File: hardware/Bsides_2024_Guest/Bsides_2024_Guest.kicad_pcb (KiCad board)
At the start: 2 copper layers, 134.5 x 127.4 mm, 45 parts, among them J1 Conn_02x03_Odd_Even, J2 Battery, J3 Battery, J4 OLED, J5 Conn_01x05, J6 Conn_01x05, P1 USB_C_Plug_USB2.0, Q1 DMG3415U-7, SW1 ON, SW2 RESET, SW3 BOOT, SW4 RESET, SW6 RESET, U1 ESP32-C6-WROOM-1U-N4, U2 AP2112K-3.3

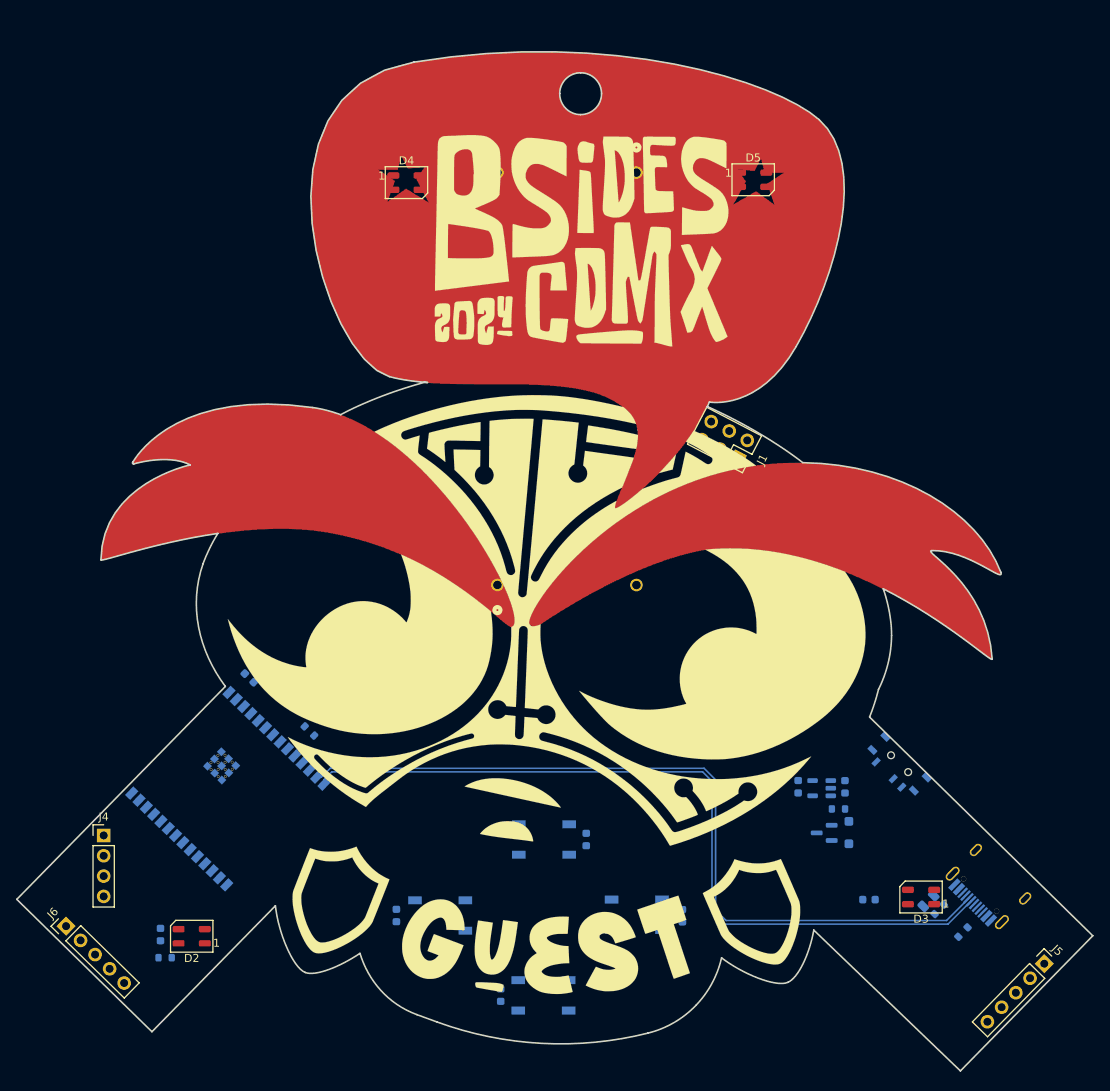
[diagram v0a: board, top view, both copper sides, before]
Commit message: feat(Hw): Update PCB
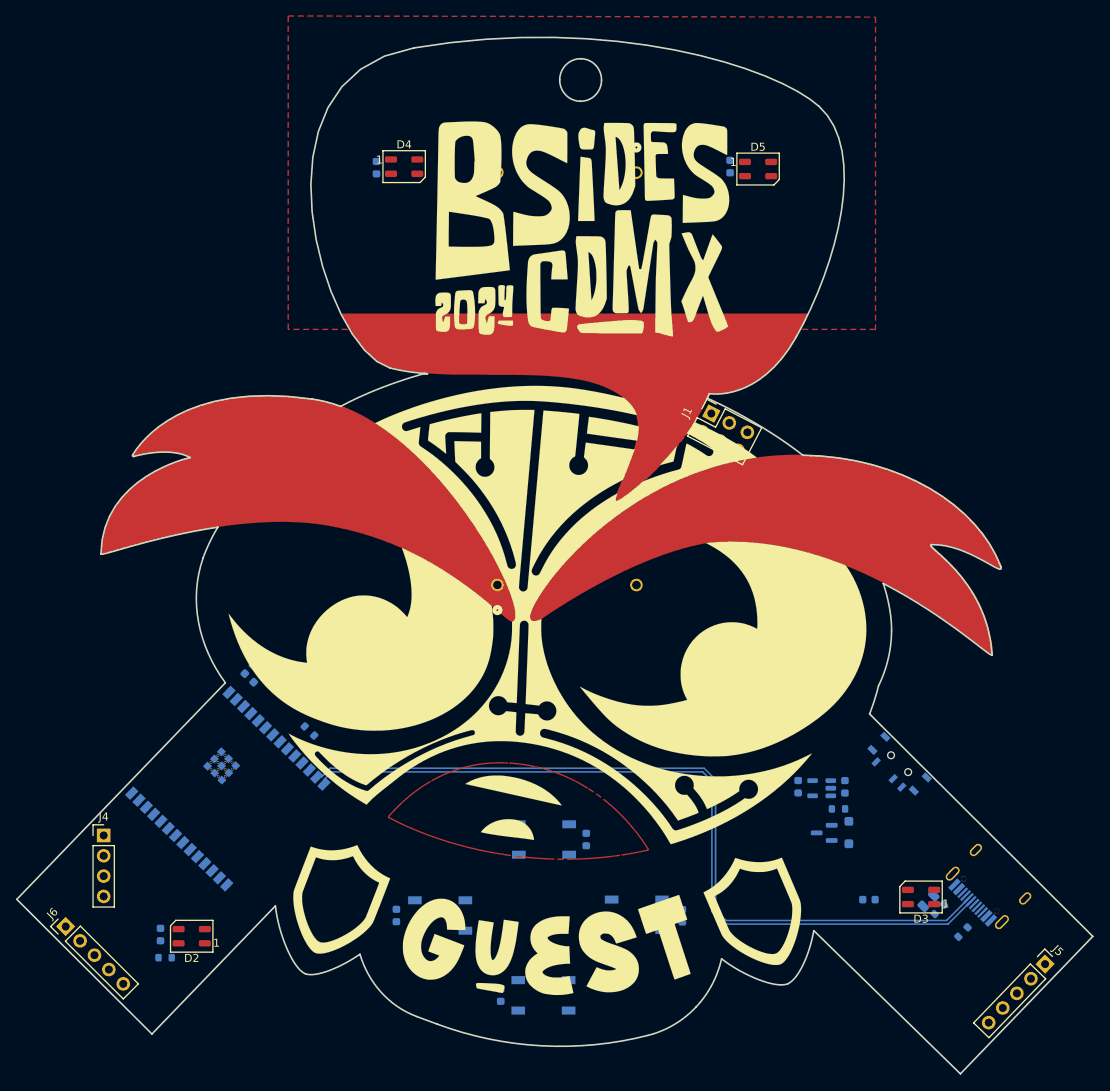
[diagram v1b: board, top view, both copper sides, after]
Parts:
- removed the Ref** at (125.5, 89.8)
- added Ref**: Val**, Guest:Badge_Guest_Bsides_2024_CDMX (1), F.Cu at (125.1, 89.3)
- J1: value Conn_02x03_Odd_Even -> Add_On
- moved J1 6.52 mm to (145.1, 71.2), turned to 62.5 degrees
- moved C7 2.02 mm to (103.2, 40.5)
- moved D4 2.02 mm to (106.7, 40.4)
- moved C12 1.47 mm to (147.4, 40.4)
- moved D5 1.47 mm to (150.9, 40.7)
- moved J5 0.11 mm to (186.8, 140.1), turned to -43.926 degrees
- moved J6 0.07 mm to (64.4, 135.4), turned to 45.111 degrees
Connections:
- C1 pad 1: Net-(SW1-B) -> VBUS
- C12 pad 2: +3V3 -> /VOUT
- C13 pad 1: +3V3 -> /VOUT
- C14 pad 1: +3V3 -> /VOUT
- C15 pad 1: +3V3 -> /VOUT
- C2 pad 1: +3V3 -> Net-(D1-A)
- C5 pad 2: +3V3 -> /VOUT
- C6 pad 2: +3V3 -> /VOUT
- C7 pad 2: +3V3 -> /VOUT
- D1 pad 2: VBUS -> Net-(D1-A)
- D2 pad 1: +3V3 -> /VOUT
- D3 pad 1: +3V3 -> /VOUT
- D4 pad 1: +3V3 -> /VOUT
- D5 pad 1: +3V3 -> /VOUT
- J1 pad 1: unconnected-(J1-Pin_1-Pad1) -> /VOUT
- J1 pad 2: unconnected-(J1-Pin_2-Pad2) -> GND
- J1 pad 3: unconnected-(J1-Pin_3-Pad3) -> /SDA
- J1 pad 4: unconnected-(J1-Pin_4-Pad4) -> /SCL
- J4 pad 1: +3V3 -> /VOUT
- Q1 pad 1: VBUS -> Net-(D1-A)
- R1 pad 2: +3V3 -> /VOUT
- R2 pad 1: VBUS -> Net-(D1-A)
- R5 pad 2: +3V3 -> /VOUT
- SW1 pad 2: Net-(SW1-B) -> /VOUT
- U1 pad 2: +3V3 -> /VOUT
- U2 pad 1: Net-(SW1-B) -> VBUS
- U2 pad 3: Net-(SW1-B) -> VBUS
- U2 pad 5: +3V3 -> Net-(D1-A)
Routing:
- added copper zone on F.Cu, net (none)
- added copper zone on F.Cu, net GND
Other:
- board size 134.5 x 127.4 mm -> 134.5 x 129.5 mm
